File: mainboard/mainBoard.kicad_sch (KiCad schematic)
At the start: 46 parts, among them J1 XT60PW-M, J2 XT60PW-M, J21 B2B-PH_K, J22 Conn_01x02, J3 XT30PW-M, J4 XT30PW-M, J5 Barrel_Jack, Q1 FQD11P06TM, Q2 FQD11P06TM, U1 TPS565208, U2 TPS565208

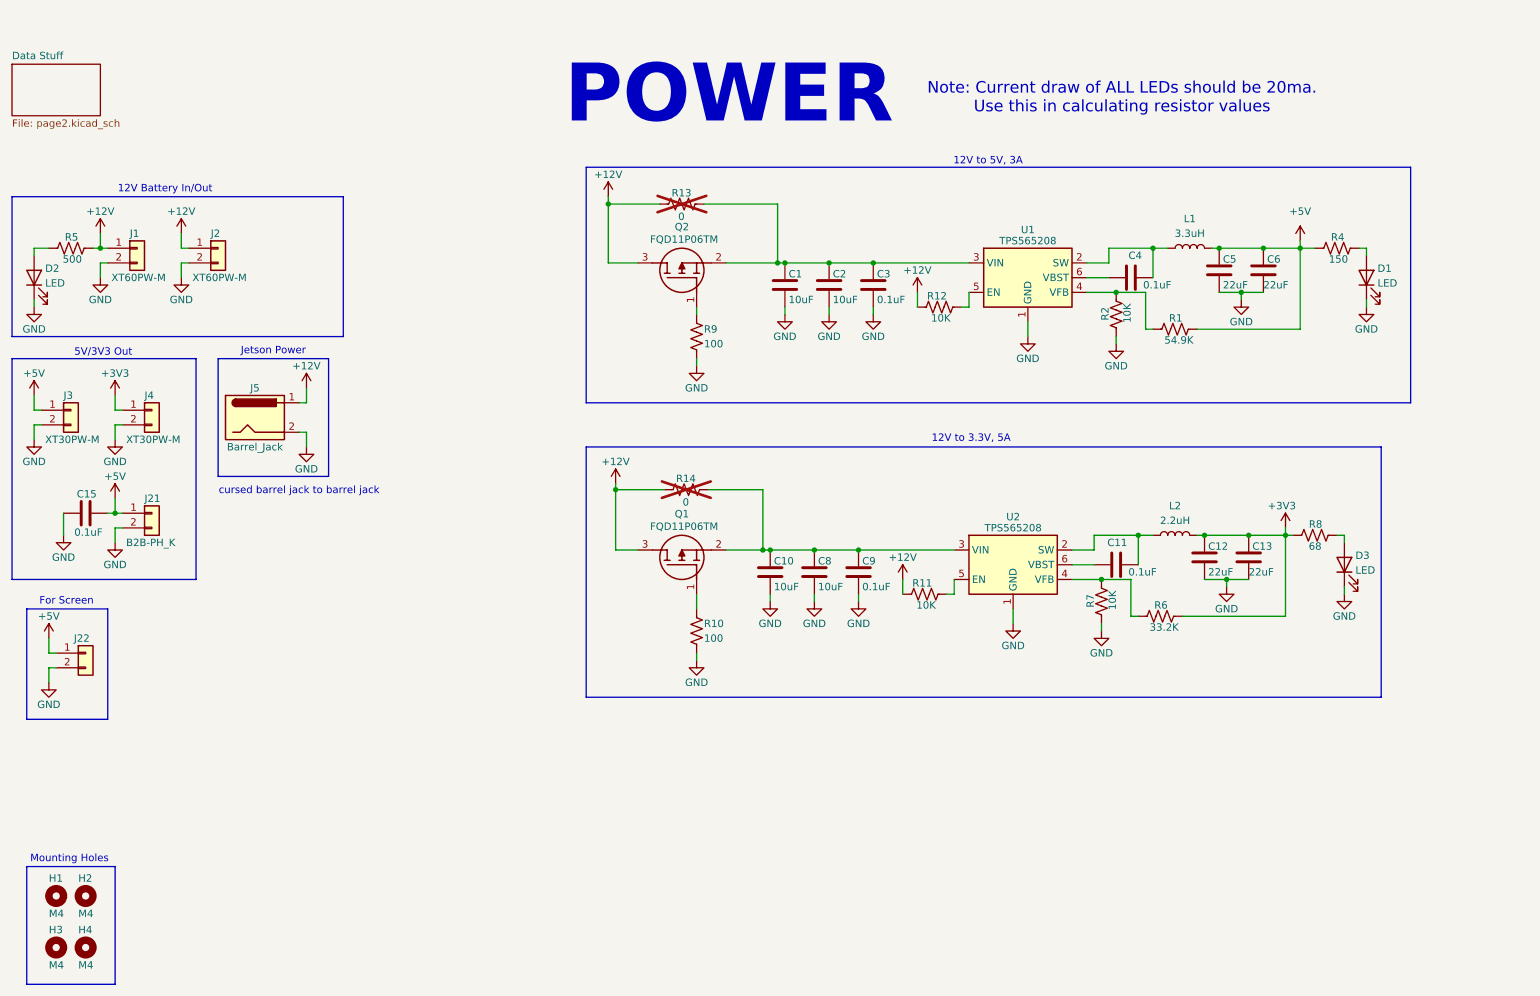
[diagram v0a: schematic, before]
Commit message: started work on mainboard
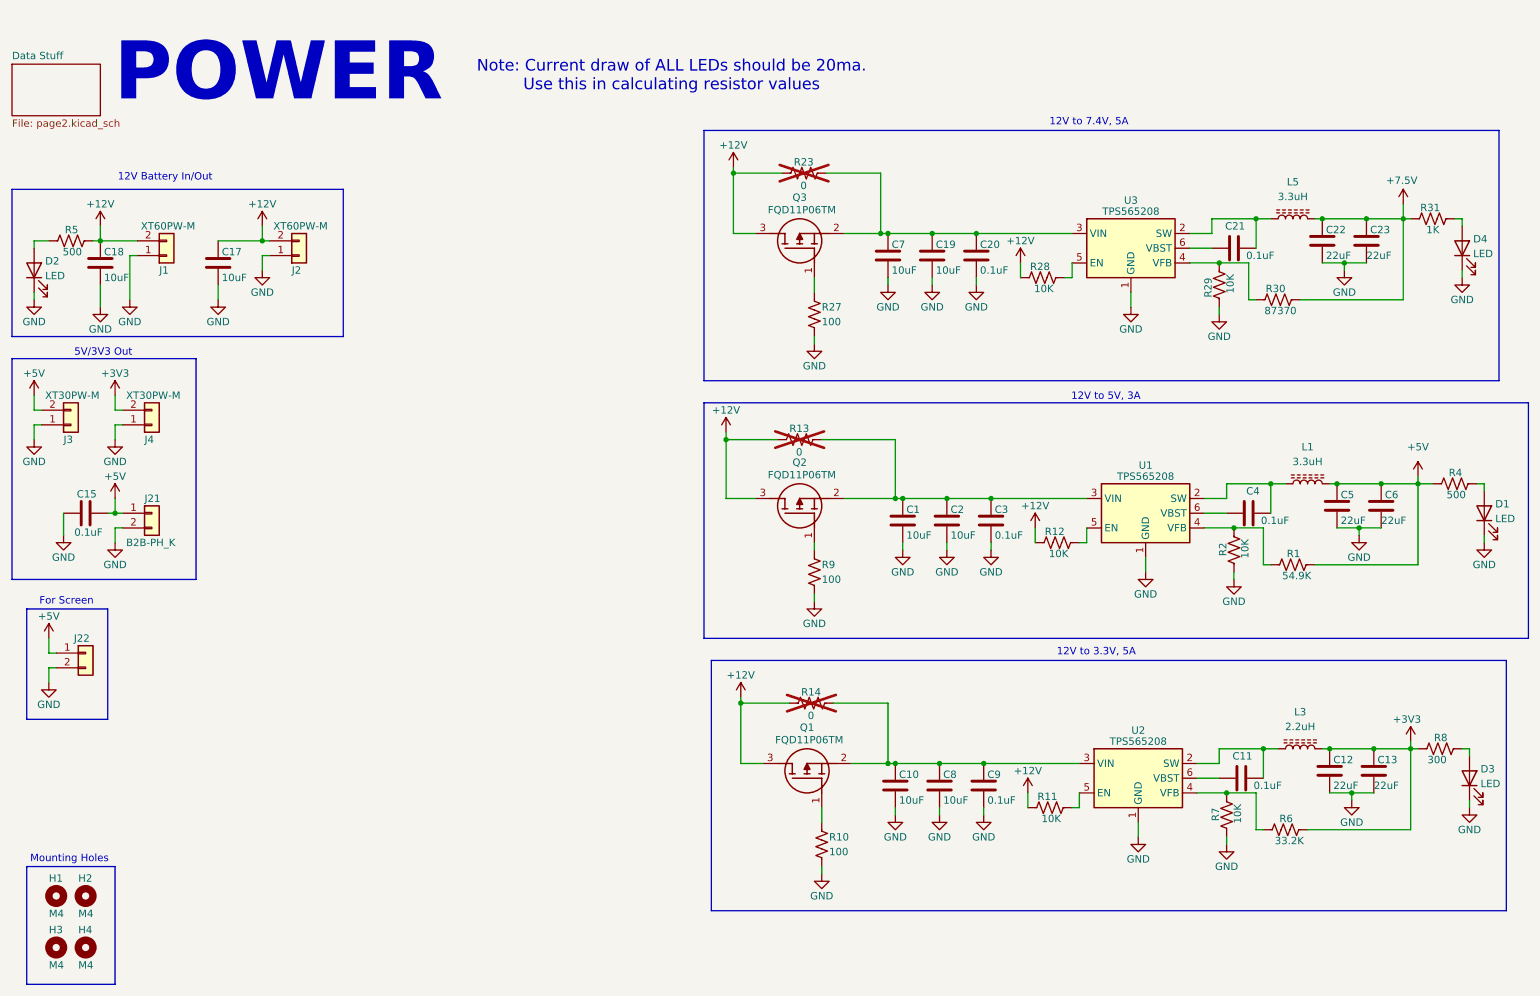
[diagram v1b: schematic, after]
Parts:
- removed J5: Barrel_Jack, Connector_BarrelJack:BarrelJack_Kycon_KLDX-0202-xC_Horizontal, symbol Connector:Barrel_Jack
- removed L1: 3.3uH, Inductor_SMD:L_Abracon_ASPI-0630LR, symbol Device:L
- removed L2: 2.2uH, Inductor_SMD:L_Abracon_ASPI-0630LR, symbol Device:L
- added C17, C18, C19, C7: 10uF, Capacitor_SMD:C_0805_2012Metric_Pad1.18x1.45mm_HandSolder, symbol Device:C
- added C20, C21: 0.1uF, Capacitor_SMD:C_0805_2012Metric_Pad1.18x1.45mm_HandSolder, symbol Device:C
- added C22, C23: 22uF, Capacitor_SMD:C_0805_2012Metric_Pad1.18x1.45mm_HandSolder, symbol Device:C
- added D4: LED, Diode_SMD:D_0805_2012Metric_Pad1.15x1.40mm_HandSolder, symbol Device:LED
- added L1, L5: 3.3uH, Inductor_SMD:L_Abracon_ASPI-0630LR, symbol Device:L_Ferrite
- added L3: 2.2uH, Inductor_SMD:L_Abracon_ASPI-0630LR, symbol Device:L_Ferrite
- added Q3: FQD11P06TM, Package_TO_SOT_SMD:TO-252-2, symbol FQD11P06TM:FQD11P06TM
- added R23: 0, Resistor_SMD:R_1210_3225Metric_Pad1.30x2.65mm_HandSolder, symbol Device:R_US
- added R27: 100, Resistor_SMD:R_0805_2012Metric_Pad1.20x1.40mm_HandSolder, symbol Device:R_US
- added R28, R29: 10K, Resistor_SMD:R_0805_2012Metric_Pad1.20x1.40mm_HandSolder, symbol Device:R_US
- added R30: 87370, Resistor_SMD:R_0805_2012Metric_Pad1.20x1.40mm_HandSolder, symbol Device:R_US
- added R31: 1K, Resistor_SMD:R_0805_2012Metric_Pad1.20x1.40mm_HandSolder, symbol Device:R_US
- added U3: TPS565208, Package_TO_SOT_SMD:SOT-23-6, symbol Regulator_Switching:TPS565208
- R4: value 150 -> 500
- R8: value 68 -> 300
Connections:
- net +12V: now also J1.2 (Pin_2), J2.2 (Pin_2), C17.1, C18.1, Q3.3 (D), R23.2, R28.1; no longer J1.1 (Pin_1), J2.1 (Pin_1)
- net +3V3: now also J4.2 (Pin_2), L3.2; no longer J4.1 (Pin_1)
- net +5V: now also J3.2 (Pin_2), L1.2; no longer J3.1 (Pin_1)
- net GND: now also J1.1 (Pin_1), J2.1 (Pin_1), J3.1 (Pin_1), J4.1 (Pin_1), C17.2, C18.2, C19.2, C20.2, C22.2, C23.2, C7.2, D4.1 (K), R27.2, R29.1, U3.1 (GND); no longer J1.2 (Pin_2), J2.2 (Pin_2), J3.2 (Pin_2), J4.2 (Pin_2)
- net at C11.2, U2.2 (SW): now also L3.1
- net at C4.2, U1.2 (SW): now also L1.1
- new net: C19.1, C20.1, C7.1, Q3.2 (S), R23.1, U3.3 (VIN)
- new net: C21.1, U3.6 (VBST)
- new net: C21.2, L5.1, U3.2 (SW)
- new net: R29.2, R30.1, U3.4 (VFB)
- new net: R28.2, U3.5 (EN)
- new net: Q3.1 (G), R27.1
- new net: D4.2 (A), R31.2
- new net +7.5V: C22.1, C23.1, L5.2, R30.2, R31.1
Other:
- note added: "12V to 7.4V, 5A"
- note removed: "Jetson Power"
- note removed: "cursed barrel jack to barrel jack"
- moved on the sheet: C1, C10, C11, C12, C13, C2, C3, C4, C5, C6, C8, C9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
